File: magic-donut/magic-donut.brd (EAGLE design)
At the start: 97.8 x 85.1 mm, 21 parts

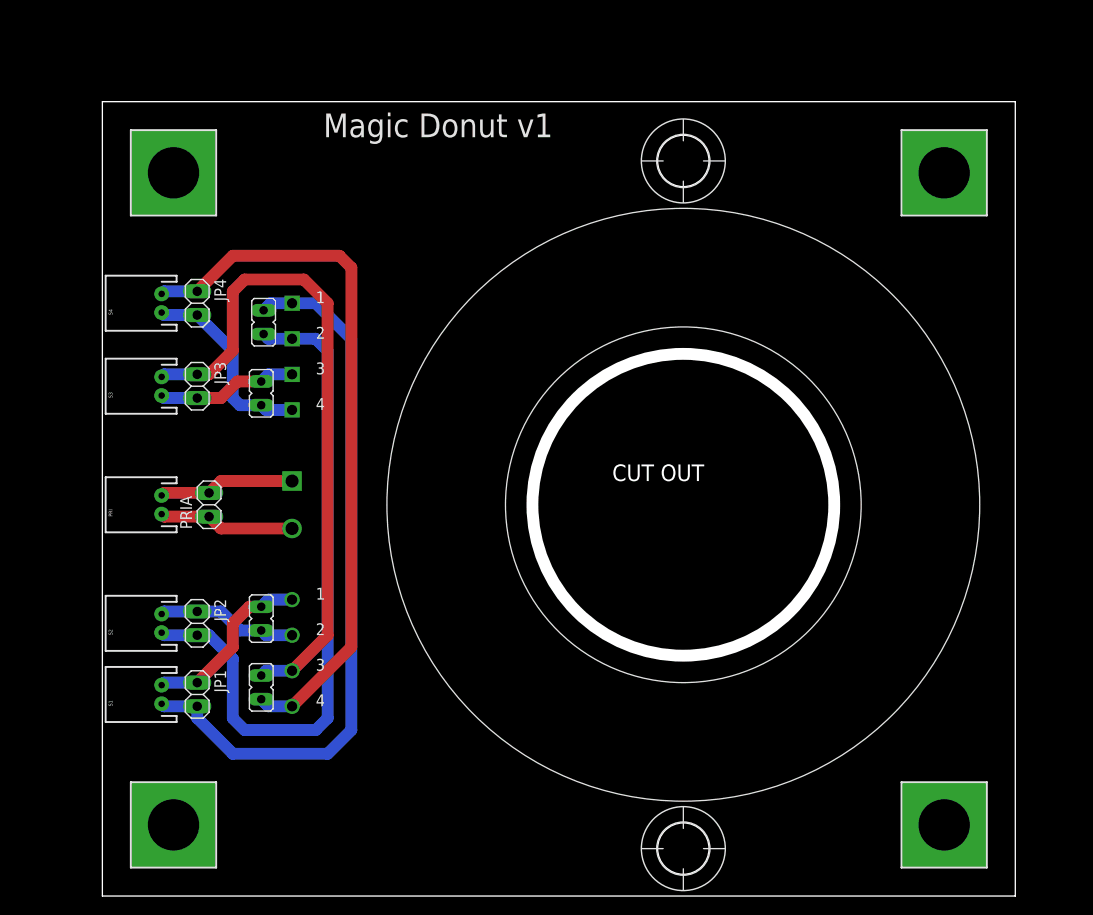
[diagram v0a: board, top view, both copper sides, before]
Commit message: wip
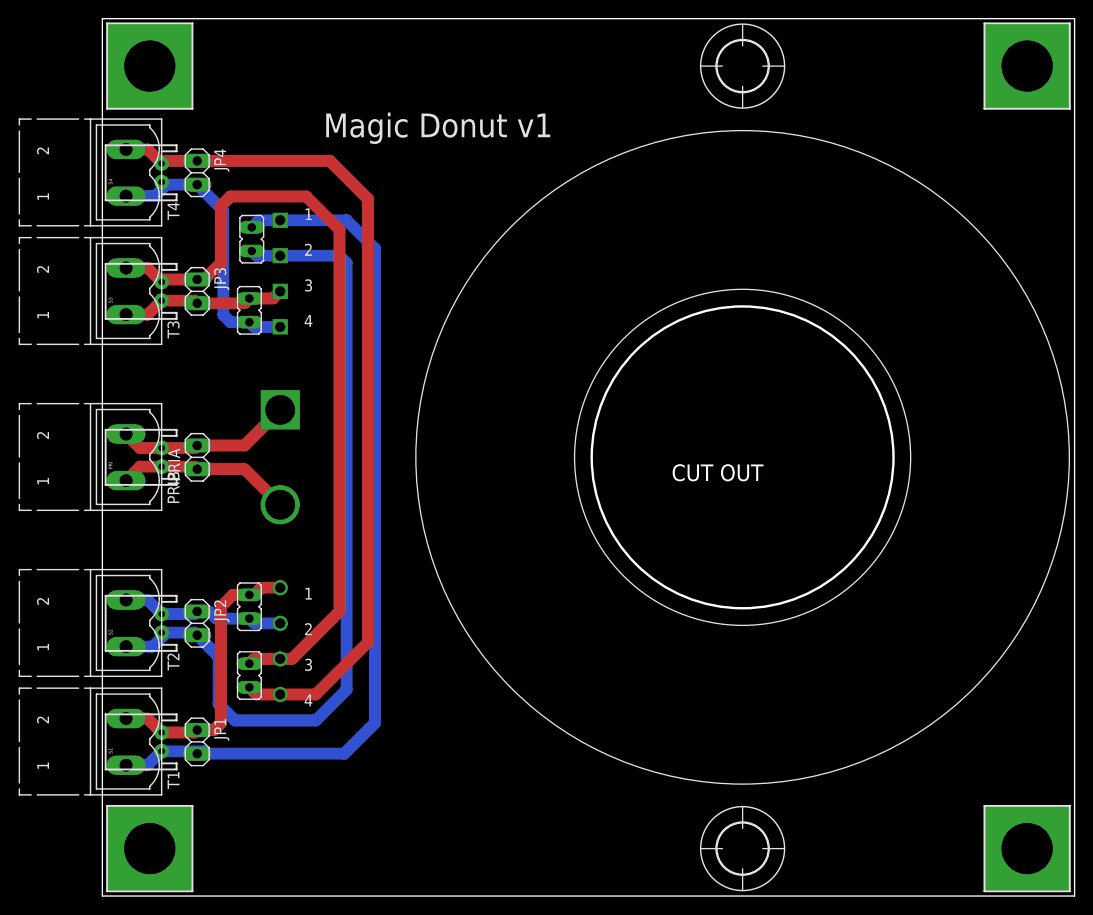
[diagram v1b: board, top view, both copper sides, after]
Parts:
- added PRIB, T1, T2, T3, T4: (no value), con-phoenix-500:MSTBV2
- moved H8 14.5 mm to (99.1, 88.9)
- moved JP4 14.0 mm to (10.2, 77.5)
- moved S4 14.0 mm to (6.35, 77.5)
- moved H1 12.0 mm to (68.6, 88.9)
- moved H6 11.7 mm to (5.08, 88.9)
- moved JP3 10.2 mm to (10.2, 64.8)
- moved S3 10.2 mm to (6.35, 64.8)
- moved H7 9.25 mm to (99.1, 5.08)
- moved BRIDGE_1_2_A 8.98 mm to (16.0, 70.4)
- moved BRIDGE_3_4_B 8.98 mm to (15.7, 62.7)
- moved U$1 8.13 mm to (68.6, 47.0)
- moved H2 6.35 mm to (68.6, 5.08)
- moved PRIA 5.24 mm to (10.2, 47.0)
- moved PRI 5.08 mm to (6.35, 47.0)
- moved JP1 5.08 mm to (10.2, 16.5)
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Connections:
- net N$1: now also T1.1
- net N$11: now also PRIB.1
- net N$12: now also PRIB.2
- net N$2: now also T2.1
- net N$3: now also T4.2
- net N$4: now also T4.1
- net N$5: now also T3.2
- net N$6: now also T3.1
- net N$7: now also T2.2
- net N$9: now also T1.2
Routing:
- net N$1: track 77.5 -> 95.9 mm
- net N$2: track 73.3 -> 89.4 mm
- net N$3: track 75.8 -> 91.2 mm
- net N$5: track 71.3 -> 85.2 mm
- net N$9: track 19.3 -> 30.8 mm
- net N$4: track 21.3 -> 30.5 mm
- net N$11: track 14.6 -> 18.8 mm
- net N$12: track 14.6 -> 18.8 mm
- net N$6: track 15.1 -> 17.8 mm
- net N$7: track 15.1 -> 17.8 mm
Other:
- board size 97.8 x 85.1 mm -> 104.1 x 94 mm
